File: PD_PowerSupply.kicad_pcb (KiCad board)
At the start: 4 copper layers, 61 x 46 mm, 81 parts, among them J1 2.54mm Header, J2 Screw Terminal, Q1 STL6P3LLH6, Q2 STL6P3LLH6, U1 LM1117LD-3.3, U2 STUSB4500QTR, U3 LMR16006YQ5, U4 LTM8074IY, U5 LTC7106EDDB-1, U6 LMP92064SDE_NOPB, U7 AQV252GAX, U8 BMD-340-A-R, U9 USB6B1

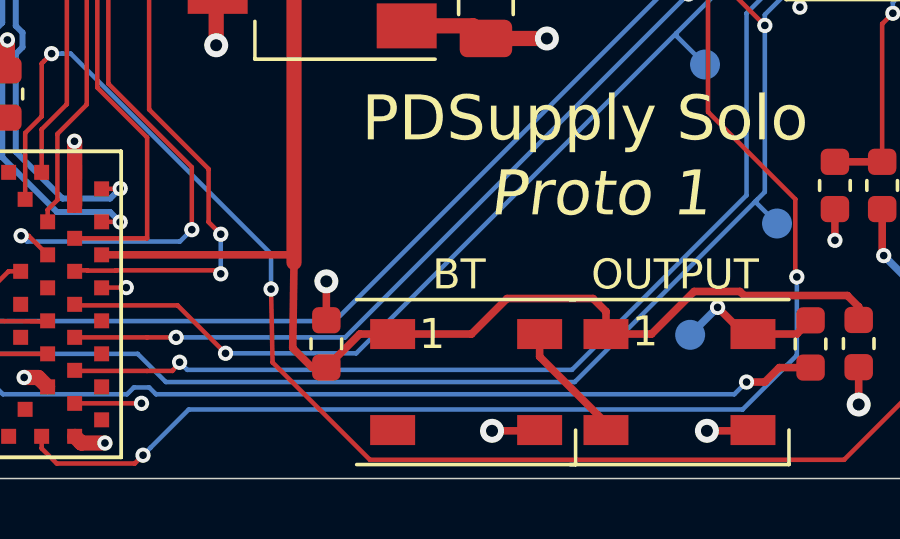
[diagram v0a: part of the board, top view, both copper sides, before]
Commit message: Regenerate Gerbers
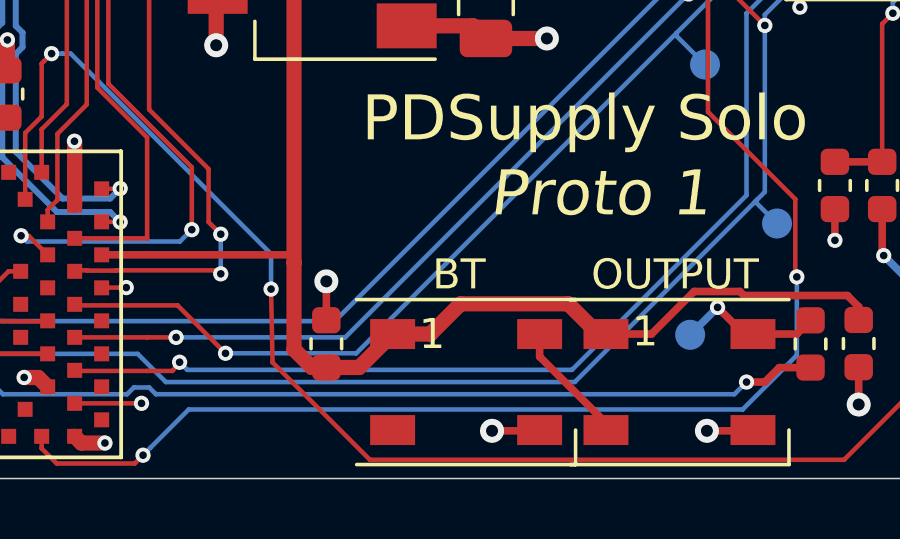
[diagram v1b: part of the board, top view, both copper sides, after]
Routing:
- net +5V: track 89.1 -> 88.5 mm
